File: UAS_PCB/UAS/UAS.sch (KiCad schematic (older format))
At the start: 17 parts, among them J1 SM02B-PASS-TBT, J2 SM02B-PASS-TBT, J3 SM02B-PASS-TBT, J4 SM02B-PASS-TBT, U1 JST-7-Pin, U10 UAS-rescue_7.5V-2.4A-Converte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, U11 JST-3-Pin, U12 Signal-Pad, U13 Signal-Pad, U2 5A-5V-Converter, U3 500mA-5V-Converter, U4 12V-StepUp-Converter, U5 TB6612FNG-Dual-Motor-Driver, U6 16_Pad_2x8_Set, U7 UAS-rescue_JST-4-Pin-UAS-cache, U8 JST-7-Pin, U9 JST-3-Pin

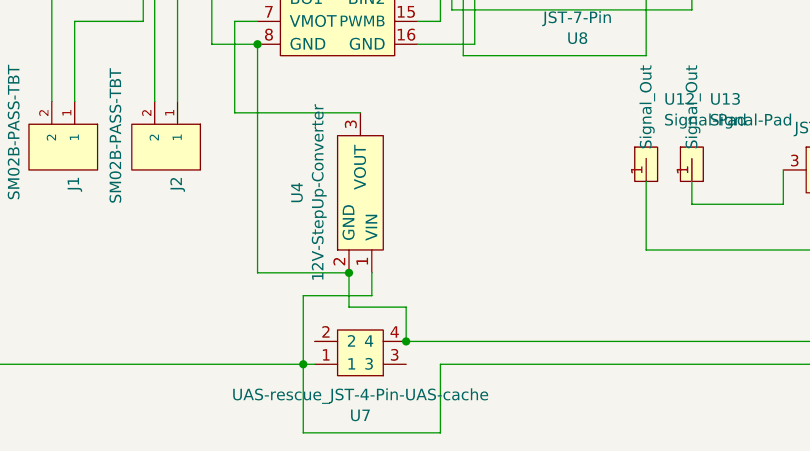
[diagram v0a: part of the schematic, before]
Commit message: First traces
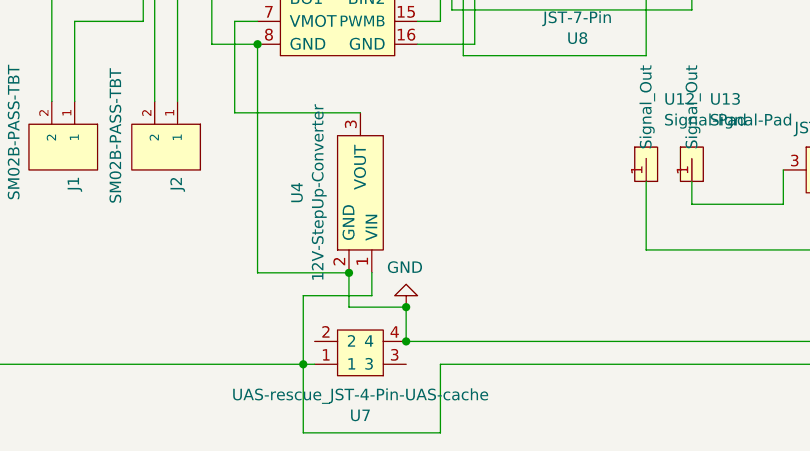
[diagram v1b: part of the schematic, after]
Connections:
- net GND: now reaches U10.4 (GND), U11.1, U2.4 (GND), U4.2 (GND), U5.8 (GND), U7.4, U9.1
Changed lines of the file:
@@
 Wire Wire Line
 	4450 5700 4450 5600
+$Comp
+L power:GND #PWR?
+U 1 1 6038ECCA
+P 3200 6150
+F 0 "#PWR?" H 3200 5900 50  0001 C CNN
+F 1 "GND" H 3205 5977 50  0000 C CNN
+F 2 "" H 3200 6150 50  0001 C CNN
+F 3 "" H 3200 6150 50  0001 C CNN
+	1    3200 6150
+	-1   0    0    1
+$EndComp
+Connection ~ 3200 6150
 $EndSCHEMATC
